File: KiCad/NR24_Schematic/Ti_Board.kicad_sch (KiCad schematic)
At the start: 3 parts, among them J5 Dash TI Connection, J6 SpeakON_NL2, J8 CAN Connector

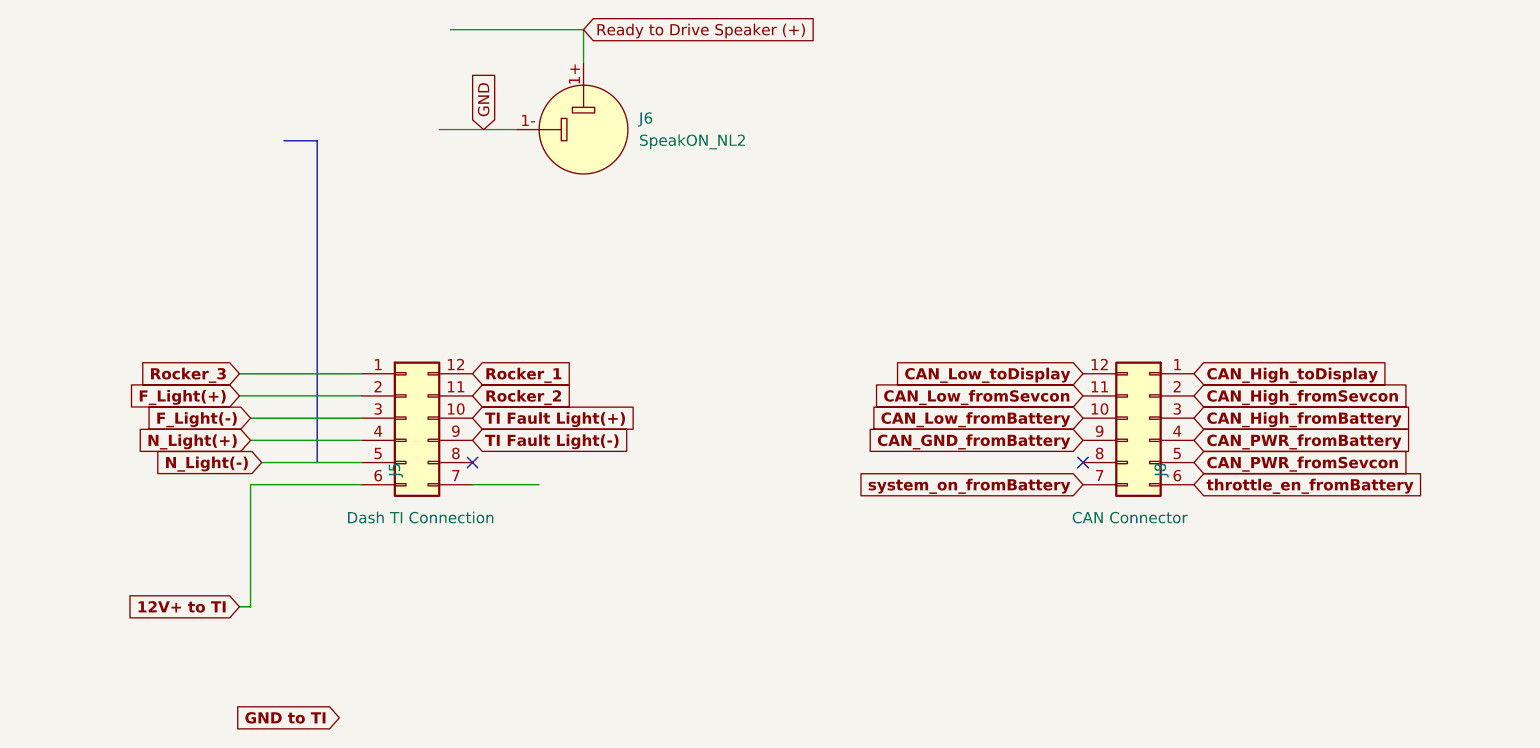
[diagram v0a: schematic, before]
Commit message: Please Finish Dash
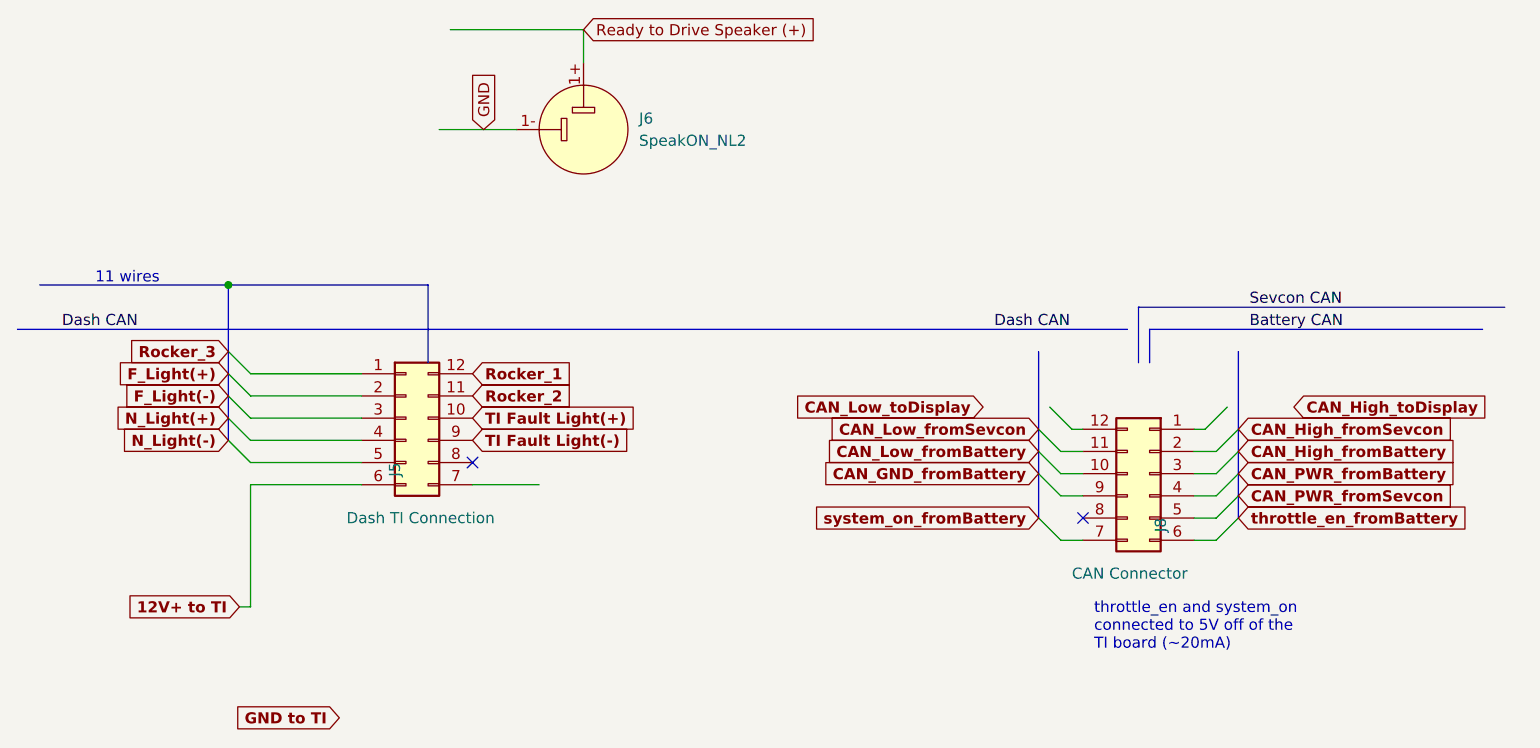
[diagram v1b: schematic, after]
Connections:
- net CAN_GND_fromBattery: no longer J8.9 (Pin_9)
- net CAN_High_fromBattery: no longer J8.3 (Pin_3)
- net CAN_High_fromSevcon: no longer J8.2 (Pin_2)
- net CAN_High_toDisplay: no longer J8.1 (Pin_1)
- net CAN_Low_fromBattery: no longer J8.10 (Pin_10)
- net CAN_Low_fromSevcon: no longer J8.11 (Pin_11)
- net CAN_Low_toDisplay: no longer J8.12 (Pin_12)
- net CAN_PWR_fromBattery: no longer J8.4 (Pin_4)
- net CAN_PWR_fromSevcon: no longer J8.5 (Pin_5)
- net F_Light(+): no longer J5.2 (Pin_2)
- net F_Light(-): no longer J5.3 (Pin_3)
- net N_Light(+): no longer J5.4 (Pin_4)
- net N_Light(-): no longer J5.5 (Pin_5)
- net Rocker_3: no longer J5.1 (Pin_1)
- net system_on_fromBattery: no longer J8.7 (Pin_7)
- net throttle_en_fromBattery: no longer J8.6 (Pin_6)
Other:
- note added: "11 wires"
- note added: "throttle_en and system_on connected to 5V off of the TI board (~20mA)"
- moved on the sheet: J8
